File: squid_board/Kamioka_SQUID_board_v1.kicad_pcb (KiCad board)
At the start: 2 copper layers, 72.1 x 111.2 mm, 18 parts, among them J1 Conn_01x25, J6 Conn_01x51

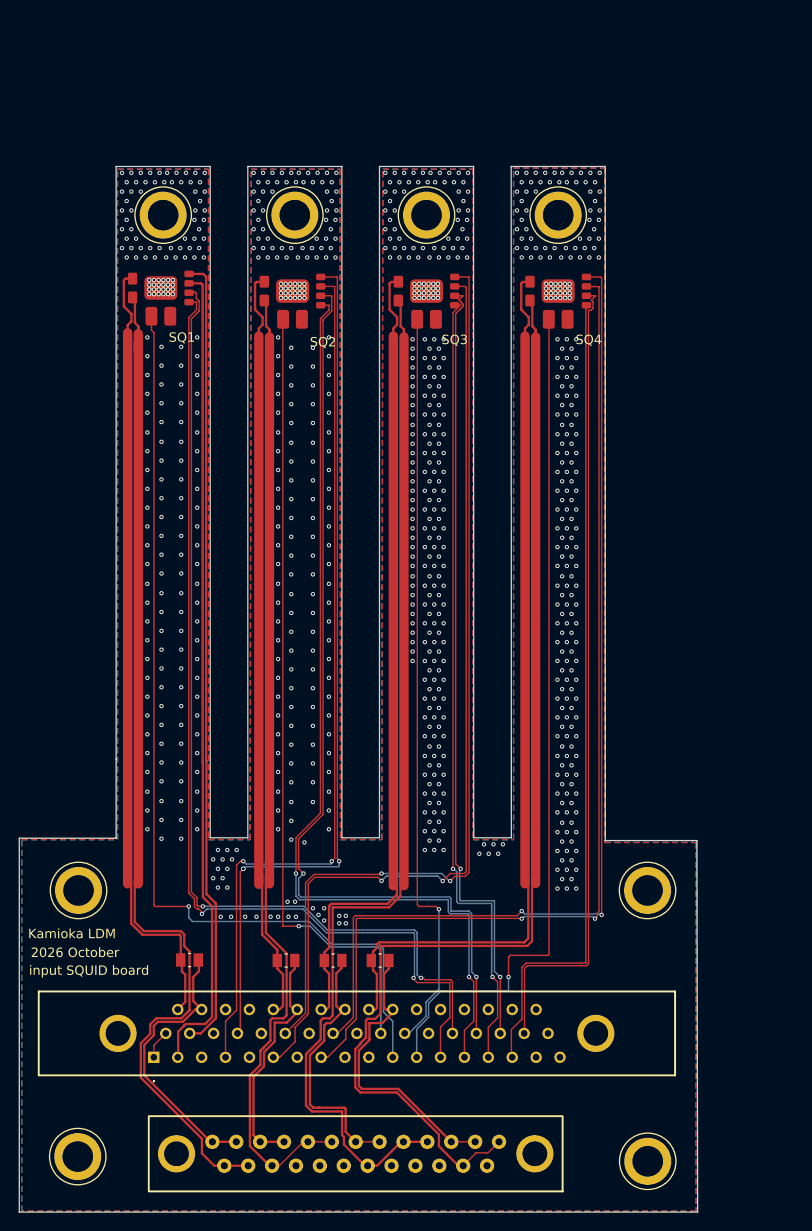
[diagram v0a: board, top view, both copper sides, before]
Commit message: add SQUID board changes
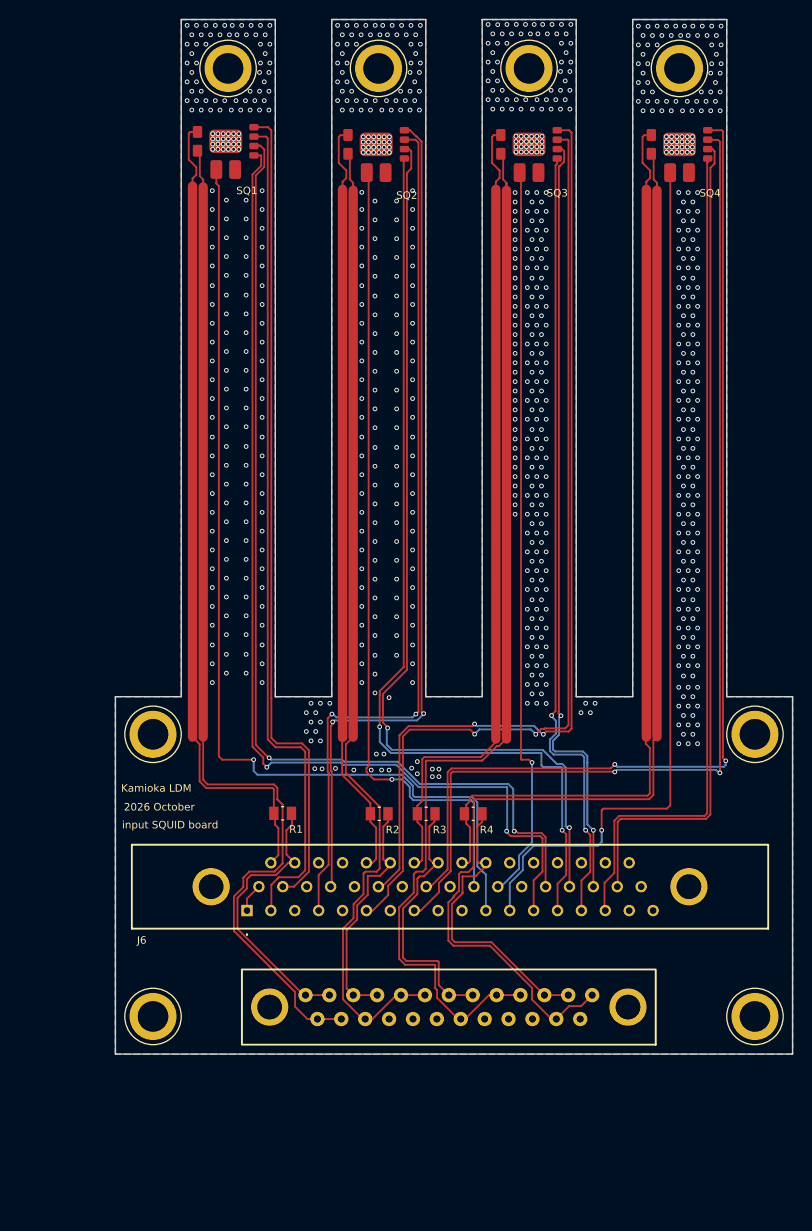
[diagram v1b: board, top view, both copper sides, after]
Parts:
- moved H7 73.5 mm to (168.0, 134.0)
- moved H6 54.8 mm to (104.0, 134.0)
- moved SQ4 20.2 mm to (160.0, 41.3)
- moved H4 20.2 mm to (160.0, 33.2)
- moved H8 20.1 mm to (168.0, 104.0)
- moved SQ3 19.0 mm to (144.0, 41.3)
- moved H3 19.0 mm to (144.0, 33.2)
- moved J1 18.5 mm to (135.4, 131.7)
- moved J6 18.5 mm to (114.0, 122.7)
- moved R2 18.5 mm to (128.0, 112.5)
- moved R3 18.5 mm to (133.0, 112.5)
- moved R1 18.5 mm to (117.8, 112.4)
- moved R4 18.5 mm to (138.0, 112.5)
- moved H5 18.4 mm to (104.0, 104.0)
- moved SQ2 18.0 mm to (127.7, 41.3)
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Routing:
- net /Ch3_3: track 118.1 -> 112.9 mm
- net /h+sq_1: track 101.7 -> 105.2 mm
- net /Ch2_3: track 107.9 -> 104.6 mm
- net /I+sq_4: track 111.0 -> 114.0 mm
- net /fb+sq_4: track 87.0 -> 89.9 mm
- net /I-sq_1: track 84.7 -> 87.5 mm
- net /I+_sq1: track 86.8 -> 89.5 mm
- net /h+sq_4: track 90.8 -> 93.4 mm
- net /fb+sq_1: track 108.0 -> 110.6 mm
- net /I-sq_4: track 109.7 -> 112.3 mm
- net /fb-sq_1: track 105.3 -> 107.7 mm
- net /b+TES1: track 84.6 -> 86.9 mm
- net /b+TES3: track 88.9 -> 86.7 mm
- net /fb-sq_4: track 86.6 -> 88.6 mm
- net /h+sq_3: track 79.7 -> 77.9 mm
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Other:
- board size 72.1 x 111.2 mm -> 72 x 110 mm
